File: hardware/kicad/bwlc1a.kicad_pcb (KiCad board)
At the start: 4 copper layers, 80 x 50 mm, 107 parts, among them J1 JST-2PH, J2 USB_C_Receptacle_USB2.0, J4 Nano SIM, J5 RSP-122811-02, Q1 DMG3415UQ-7, Q2 NPN, Q3 NPN, Q4 NPN, Q5 NPN, Q6 NPN, SW1 EN_ESP, U1 MCP73831-2-OT, U2 USBLC6-2SC6, U3 TPS62290DRVR, U4 MAX17048G+, U5 LSM6DS3, U6 ESP32-S3-MINI-1, U7 L86-M33, U8 MIC29302WU, U9 A7670C_24x24mm, Y1 32.768 kHz

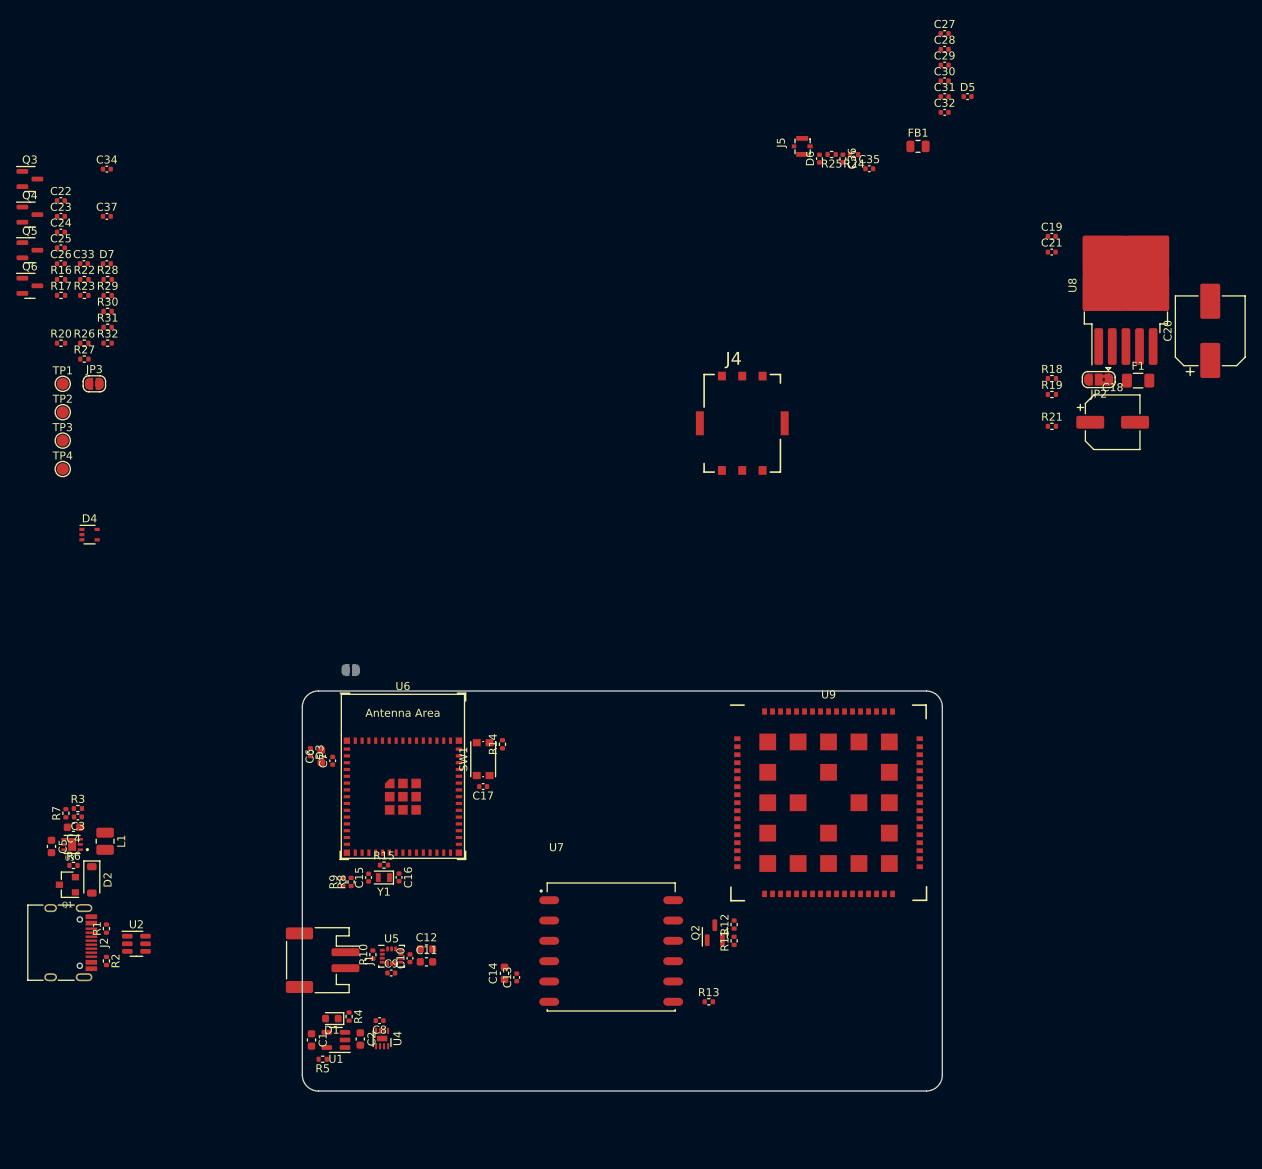
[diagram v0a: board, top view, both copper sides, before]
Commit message: Update on PCB Layout
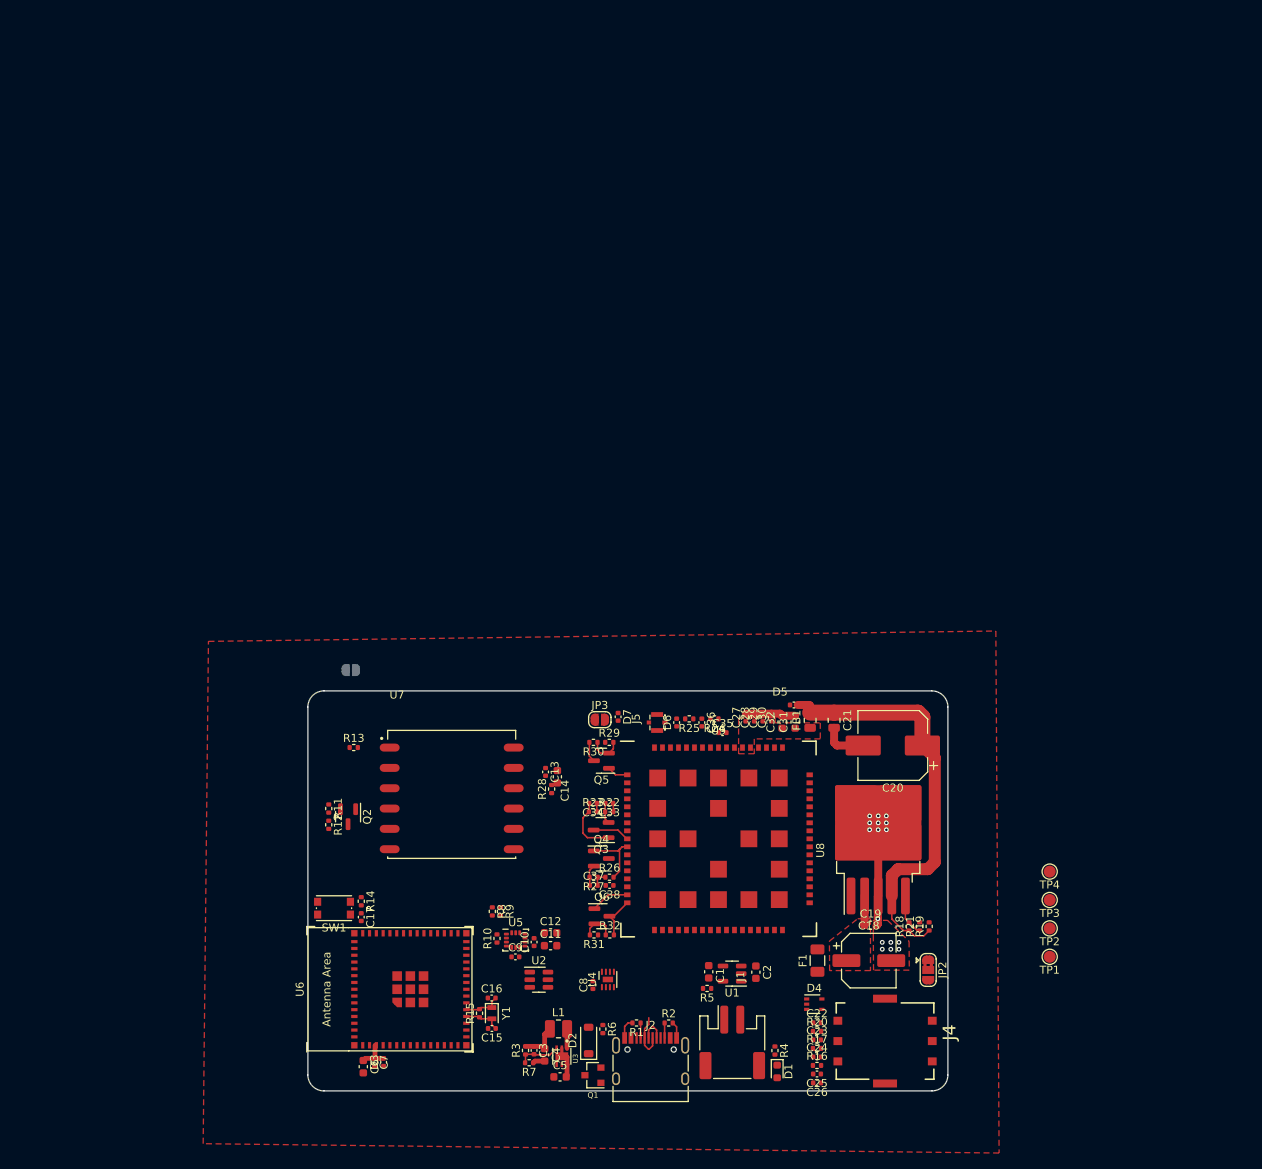
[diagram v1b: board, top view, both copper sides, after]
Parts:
- added C38: 100n, Capacitor_SMD:C_0402_1005Metric, F.Cu at (142.8, 102.9)
- C19, C31, C32: footprint Capacitor_SMD:C_0402_1005Metric -> Capacitor_SMD:C_0603_1608Metric
- C21: footprint Capacitor_SMD:C_0402_1005Metric -> Capacitor_SMD:C_0805_2012Metric
- moved TP1 142.7 mm to (197.8, 111.8), turned to 180 degrees
- moved C25 140.0 mm to (168.7, 126.5), turned to 180 degrees
- moved C24 139.9 mm to (168.7, 124.4)
- moved C23 139.7 mm to (168.7, 122.2)
- moved C22 139.6 mm to (168.7, 120.1)
- moved C26 139.4 mm to (168.7, 127.6), turned to 180 degrees
- moved TP2 139.2 mm to (197.8, 108.3), turned to 180 degrees
- moved R16 136.3 mm to (168.7, 125.4)
- moved TP3 136.1 mm to (197.8, 104.7), turned to 180 degrees
- moved R17 133.4 mm to (168.7, 123.3)
- moved TP4 133.2 mm to (197.8, 101.2), turned to 180 degrees
- moved R20 127.8 mm to (168.7, 121.2)
- moved Q3 108.3 mm to (141.7, 96.0), turned to 180 degrees
- moved D4 107.9 mm to (168.4, 117.8)
- moved Q4 107.6 mm to (141.8, 99.6)
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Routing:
- net VDD_BAT: track 0.00 -> 53.8 mm
- net GND: track 0.00 -> 43.2 mm, vias 0 -> 16
- net IMU_VDD: track 0.00 -> 10.6 mm
- net A7670_UART_RX: track 0.00 -> 8.17 mm
- net A7670_TX: track 0.00 -> 7.50 mm
- net USB_D-: track 0.00 -> 6.03 mm
- net /TPS_FB: track 0.00 -> 5.30 mm
- net Net-(U8-ADJ): track 0.00 -> 5.23 mm
- net ESP_32K_P: track 0.00 -> 4.91 mm
- net ESP_32K_N: track 0.00 -> 4.85 mm
- net RESET: track 0.00 -> 4.82 mm
- net A7670_UART_TX: track 0.00 -> 4.66 mm
- net Net-(Q6-B): track 0.00 -> 4.29 mm
- net Net-(Q5-B): track 0.00 -> 4.12 mm
- net Net-(JP2-A): track 0.00 -> 3.68 mm
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- added copper zone on F.Cu, net GND
- added copper zone on In1.Cu, net GND
- added copper zone on F.Cu, net Net-(C27-Pad1)
- added copper zone on F.Cu, net Net-(JP2-A)
